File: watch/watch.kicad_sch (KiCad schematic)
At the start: 26 parts, among them SW1 ButtonWakeup, SW2 ButtonUp, SW3 ButtonDown, U1 STM32L031F4Px, Y1 CR_32kHz

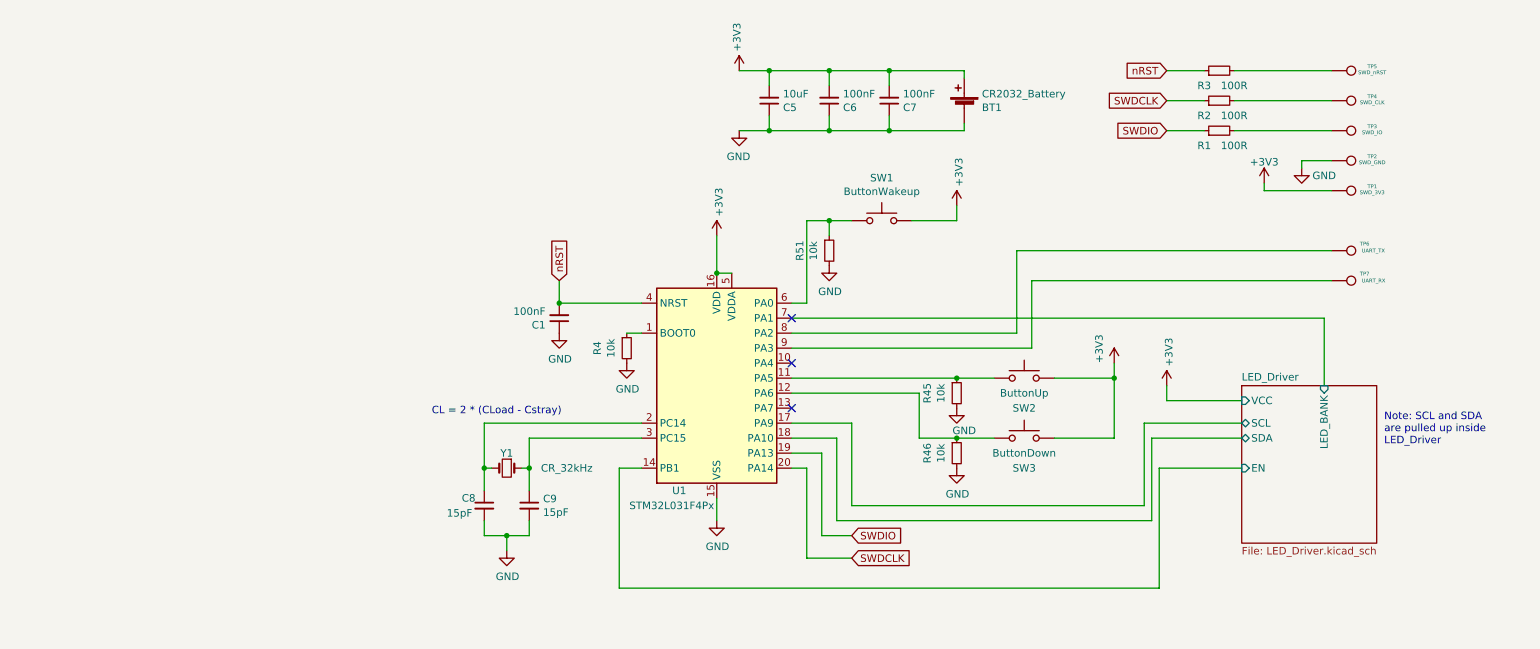
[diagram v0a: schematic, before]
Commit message: as ordered V1.4
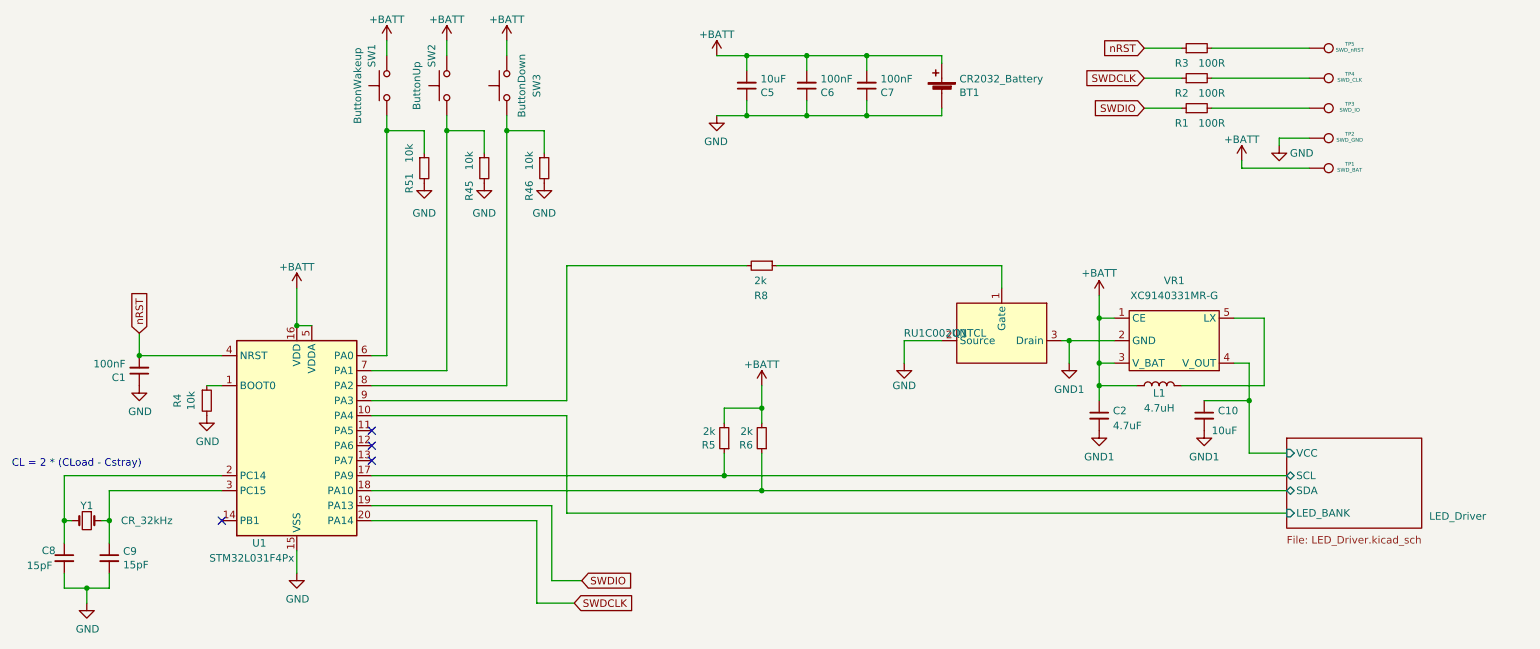
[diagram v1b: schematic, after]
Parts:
- removed TP6: UART_TX, TestPoint:TestPoint_Pad_D2.0mm, symbol Connector:TestPoint
- removed TP7: UART_RX, TestPoint:TestPoint_Pad_D2.0mm, symbol Connector:TestPoint
- added C10: 10uF, custom:C_0603_1608Metric, symbol Device:C_Small
- added C2: 4.7uF, custom:C_0603_1608Metric, symbol Device:C_Small
- added L1: 4.7uH, Inductor_SMD:L_0603_1608Metric_Pad1.05x0.95mm_HandSolder, symbol Device:L
- added Q1: RU1C002UNTCL, mrab:SOT-323FL, symbol custom:RU1C002UNTCL
- added R5, R6, R8: 2k, custom:R_0603_1608Metric, symbol Device:R_Small
- added VR1: XC9140331MR-G, mrab:SOT-25, symbol custom:XC9140331MR-G
- BT1: footprint BAT-HLD-001:BATHLD001 -> SamacSys_Parts:BATHLD001
- TP1: value SWD_3V3 -> SWD_BAT
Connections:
- net GND: now also Q1.2 (Source)
- net LED_Driver/LED_BANK: now also U1.10 (PA4); no longer U1.7 (PA1)
- net LED_Driver/SCL: now also R5.1
- net LED_Driver/SDA: now also R6.1
- net at R45.1, SW2.1: now also U1.7 (PA1); no longer U1.11 (PA5)
- net at R46.1, SW3.1: now also U1.8 (PA2); no longer U1.12 (PA6)
- net at U1.9 (PA3): now also R8.2
- net +3V3 renamed +BATT
- net +BATT: now also C2.1, L1.1, R5.2, R6.2, VR1.1 (CE), VR1.3 (V_BAT)
- net LED_Driver/EN: no longer names the net of U1.14 (PB1)
- new net: L1.2, VR1.5 (LX)
- new net: Q1.1 (Gate), R8.1
- new net GND1: C10.2, C2.2, Q1.3 (Drain), VR1.2 (GND)
- new net LED_Driver/VCC: C10.1, VR1.4 (V_OUT)
- no-connect marks 3 -> 4
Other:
- sheet LED_Driver ports: added none; removed EN
- note removed: "Note: SCL and SDA are pulled up inside LED_Driver"
- moved on the sheet: BT1, C1, C5, C6, C7, C8, C9, R1, R2, R3, R4, R45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
